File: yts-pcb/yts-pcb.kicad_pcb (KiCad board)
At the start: 2 copper layers, 210 x 78 mm, 62 parts, among them J1 B+, J2 B-, SW1 ON/OFF, SW10 MX, SW11 MX, SW12 MX, SW13 MX, SW14 MX, SW15 MX, SW16 MX, SW17 MX, SW18 MX, SW19 MX, SW2 MX, SW20 MX, SW21 MX, SW22 MX, SW23 MX, SW24 MX, SW25 MX, SW26 MX, SW27 MX, SW28 MX, SW29 RotaryEncoder_Switch, SW3 MX, SW30 RotaryEncoder_Switch, SW4 MX, SW5 MX, SW6 MX, SW7 MX, SW8 MX, SW9 MX, U1 Nice!Nano

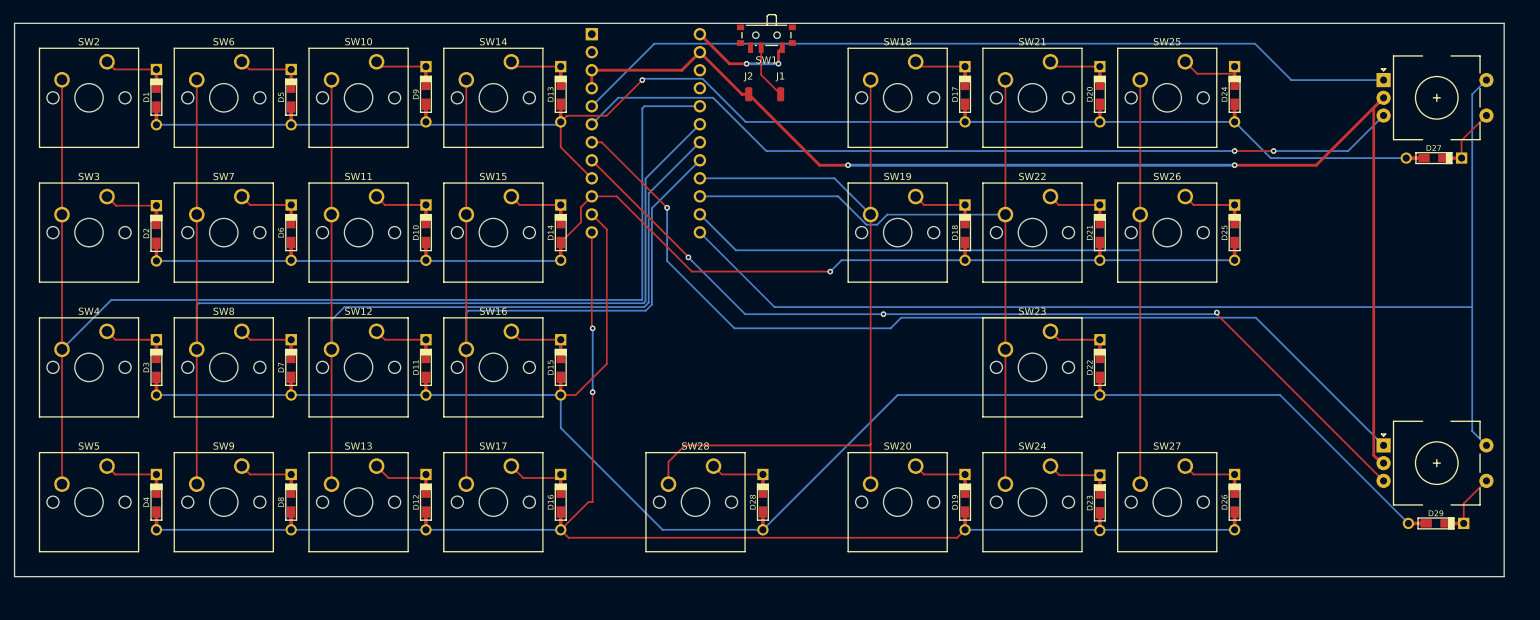
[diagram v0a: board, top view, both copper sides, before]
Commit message: update switchblade
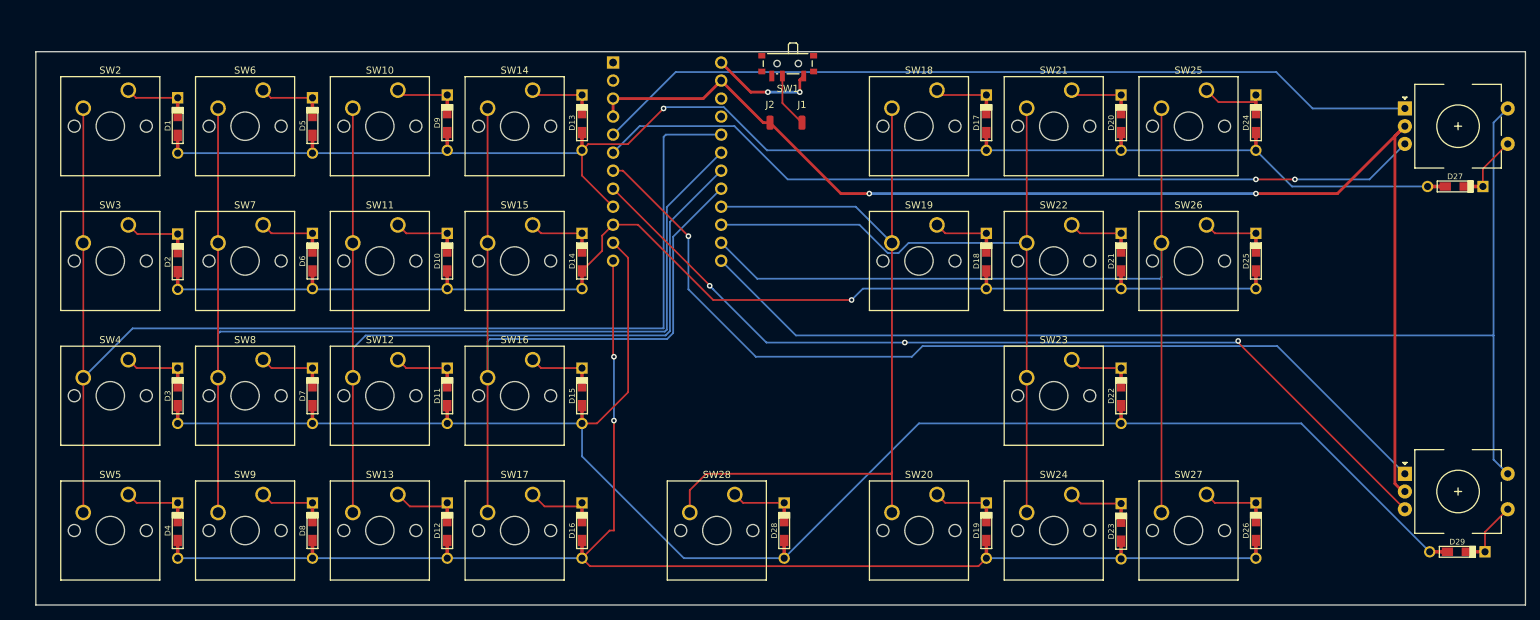
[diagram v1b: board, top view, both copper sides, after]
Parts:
- moved D1 5.00 mm to (60.0, 51.4)
- moved D10 5.00 mm to (98.0, 70.5)
- moved D11 5.00 mm to (98.0, 89.5)
- moved D12 5.00 mm to (98.0, 108.5)
- moved D13 5.00 mm to (117.0, 51.0)
- moved D14 5.00 mm to (117.0, 70.5)
- moved D15 5.00 mm to (117.0, 89.5)
- moved D16 5.00 mm to (117.0, 108.5)
- moved D17 5.00 mm to (174.0, 51.0)
- moved D18 5.00 mm to (174.0, 70.5)
- moved D19 5.00 mm to (174.0, 108.5)
- moved D2 5.00 mm to (60.0, 70.6)
- moved D20 5.00 mm to (193.0, 51.0)
- moved D21 5.00 mm to (193.0, 70.5)
- moved D22 5.00 mm to (193.0, 89.5)
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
